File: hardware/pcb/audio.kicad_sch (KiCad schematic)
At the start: 10 parts, among them IC3 TAC5212, J4 PJ-342, J5 PJ-242

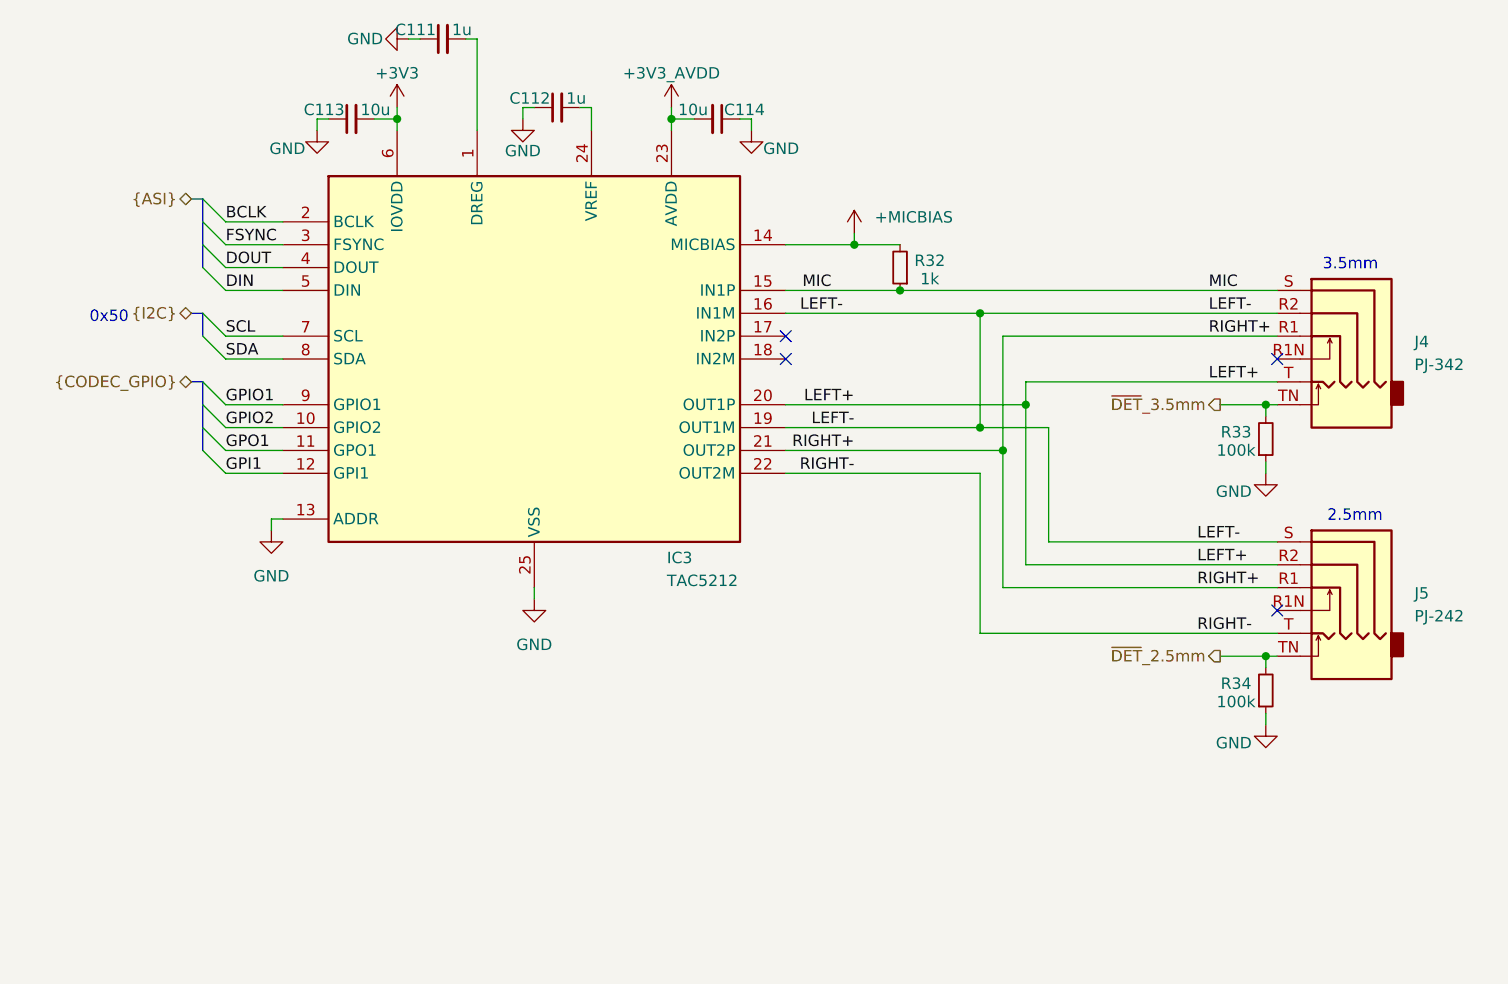
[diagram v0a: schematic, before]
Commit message: added a bunch testpoints
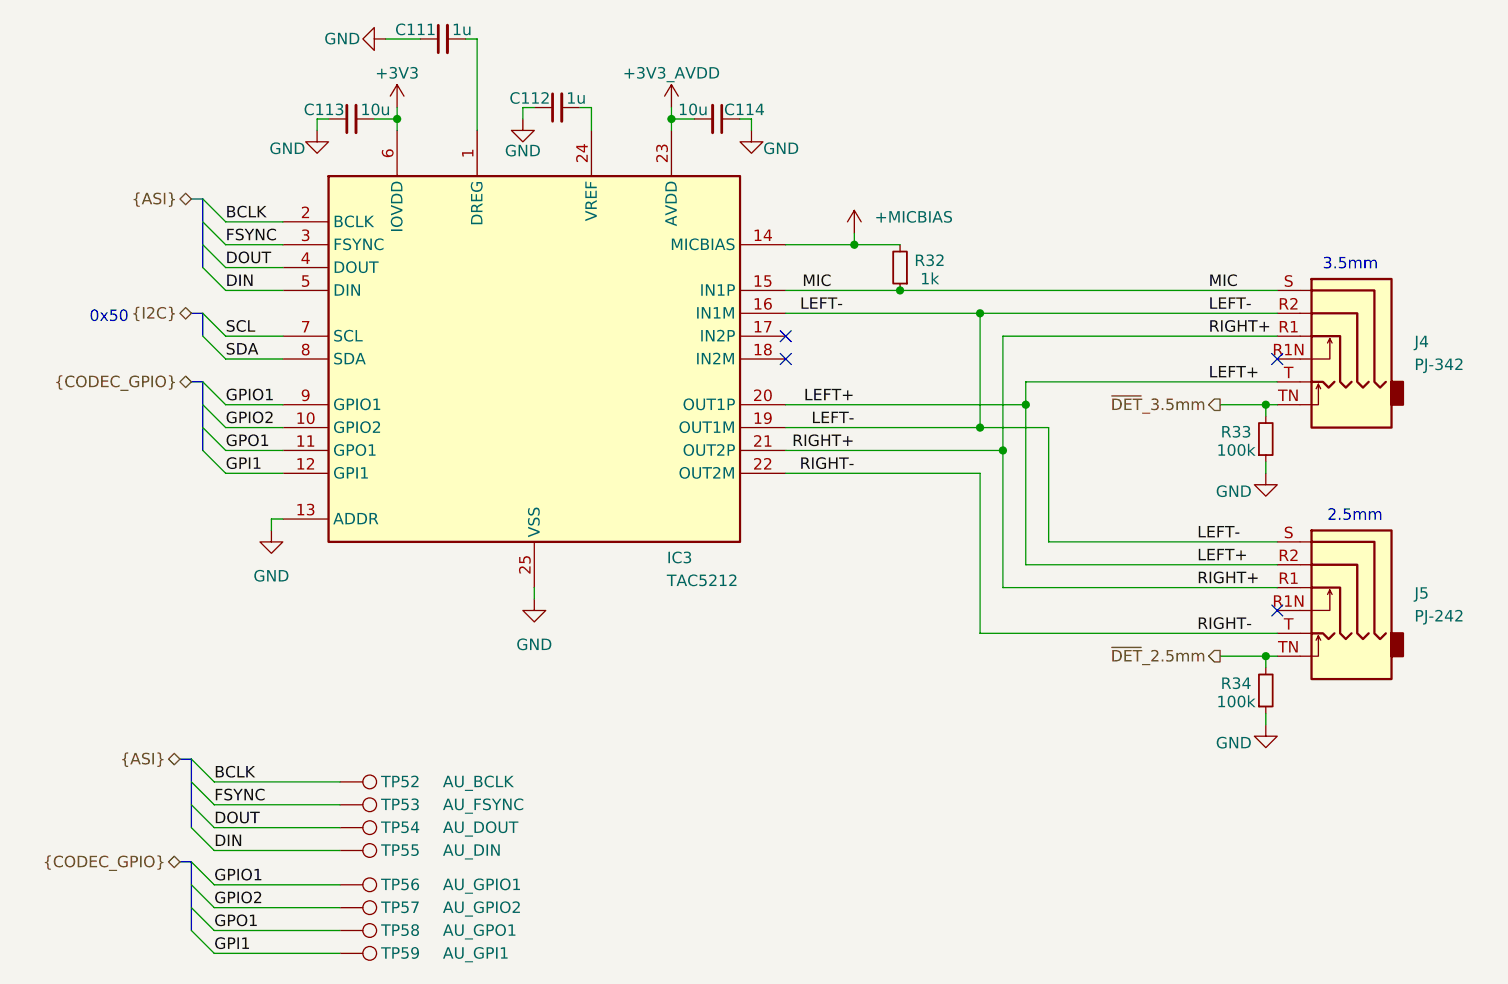
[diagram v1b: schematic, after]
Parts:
- added TP52: AU_BCLK, TestPoint:TestPoint_Pad_D1.0mm, symbol Connector:TestPoint
- added TP53: AU_FSYNC, TestPoint:TestPoint_Pad_D1.0mm, symbol Connector:TestPoint
- added TP54: AU_DOUT, TestPoint:TestPoint_Pad_D1.0mm, symbol Connector:TestPoint
- added TP55: AU_DIN, TestPoint:TestPoint_Pad_D1.0mm, symbol Connector:TestPoint
- added TP56: AU_GPIO1, TestPoint:TestPoint_Pad_D1.0mm, symbol Connector:TestPoint
- added TP57: AU_GPIO2, TestPoint:TestPoint_Pad_D1.0mm, symbol Connector:TestPoint
- added TP58: AU_GPO1, TestPoint:TestPoint_Pad_D1.0mm, symbol Connector:TestPoint
- added TP59: AU_GPI1, TestPoint:TestPoint_Pad_D1.0mm, symbol Connector:TestPoint
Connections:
- net BCLK: now also TP52.1
- net DIN: now also TP55.1
- net DOUT: now also TP54.1
- net FSYNC: now also TP53.1
- net GPI1: now also TP59.1
- net GPIO1: now also TP56.1
- net GPIO2: now also TP57.1
- net GPO1: now also TP58.1
